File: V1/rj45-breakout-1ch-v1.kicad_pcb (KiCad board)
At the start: 2 copper layers, 22 x 28 mm, 2 parts, among them J1 RJ45, J2 1x4P 5,08 SCREW

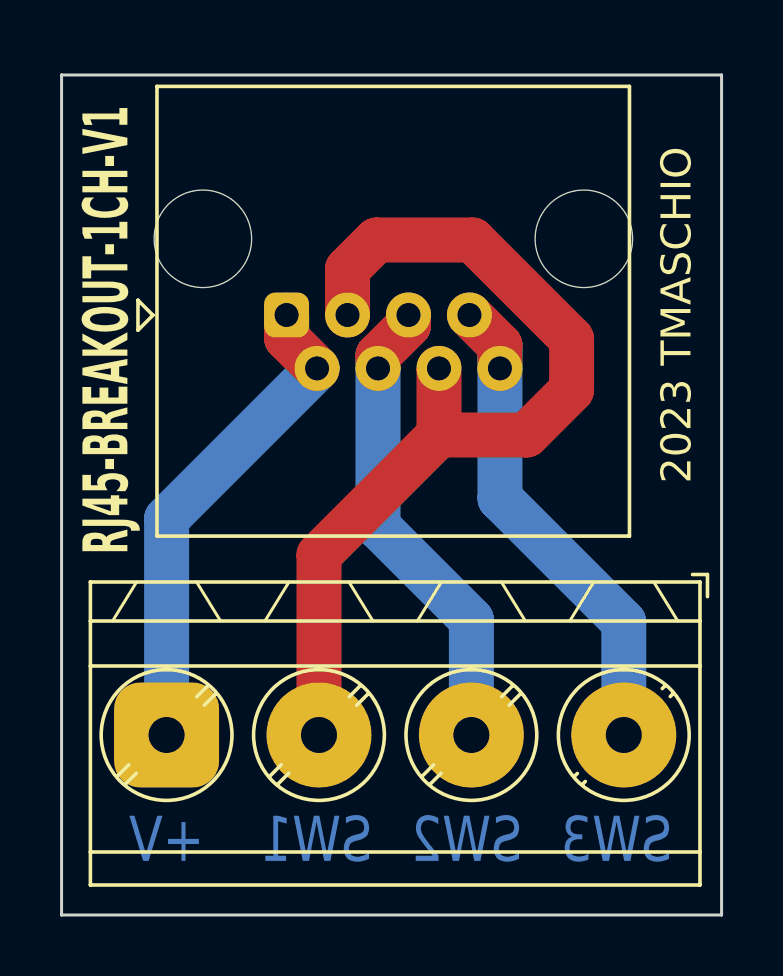
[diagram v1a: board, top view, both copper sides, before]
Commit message: Adjusting before fabrication
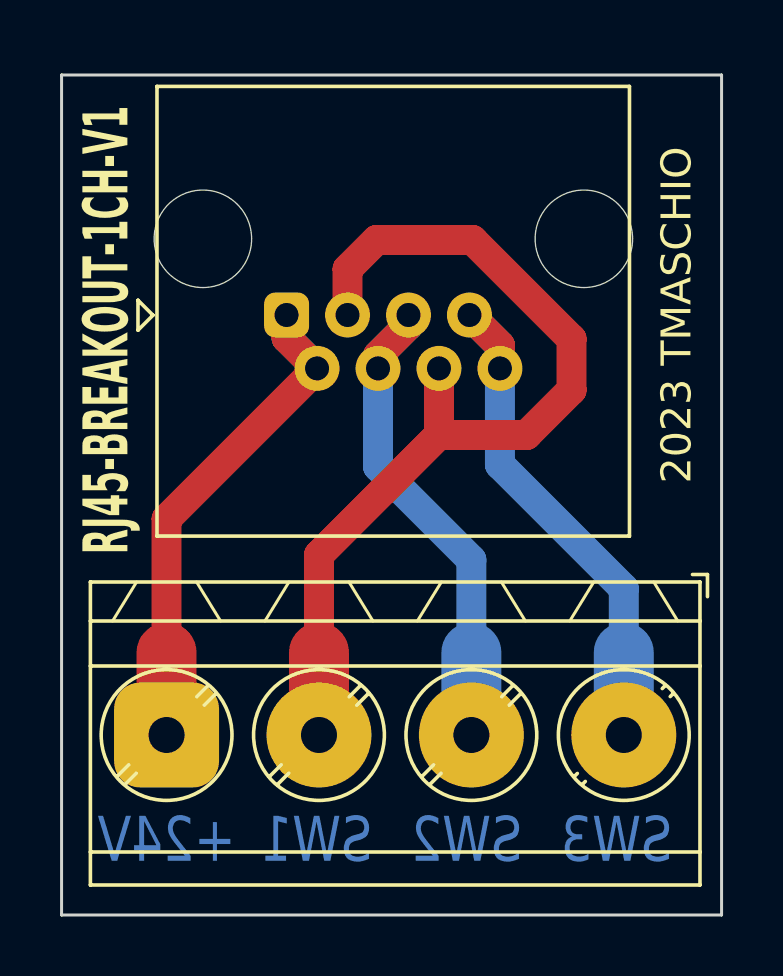
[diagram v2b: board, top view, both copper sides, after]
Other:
- rule pad_to_mask_clearance: 0 -> 0.1
- board text added: "+24V"
- board text removed: "+V"
